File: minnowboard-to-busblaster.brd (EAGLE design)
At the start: 72.4 x 35.6 mm, 19 parts, among them J1 CIRCUITCO_MINNOW2_HIGH_SPEED, U1 SN74LV4T125, U2 SN74LV1T125, U3 SN74LV1T125

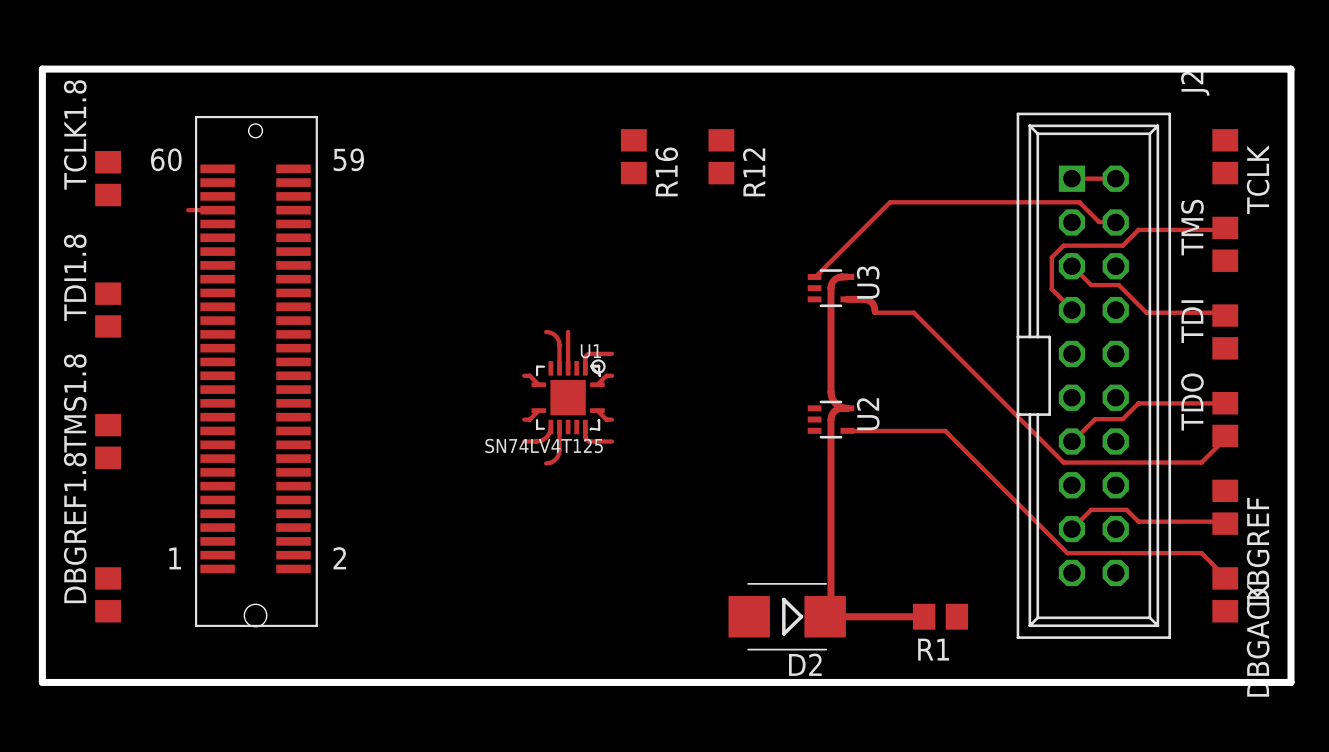
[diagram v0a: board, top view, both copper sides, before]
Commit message: all
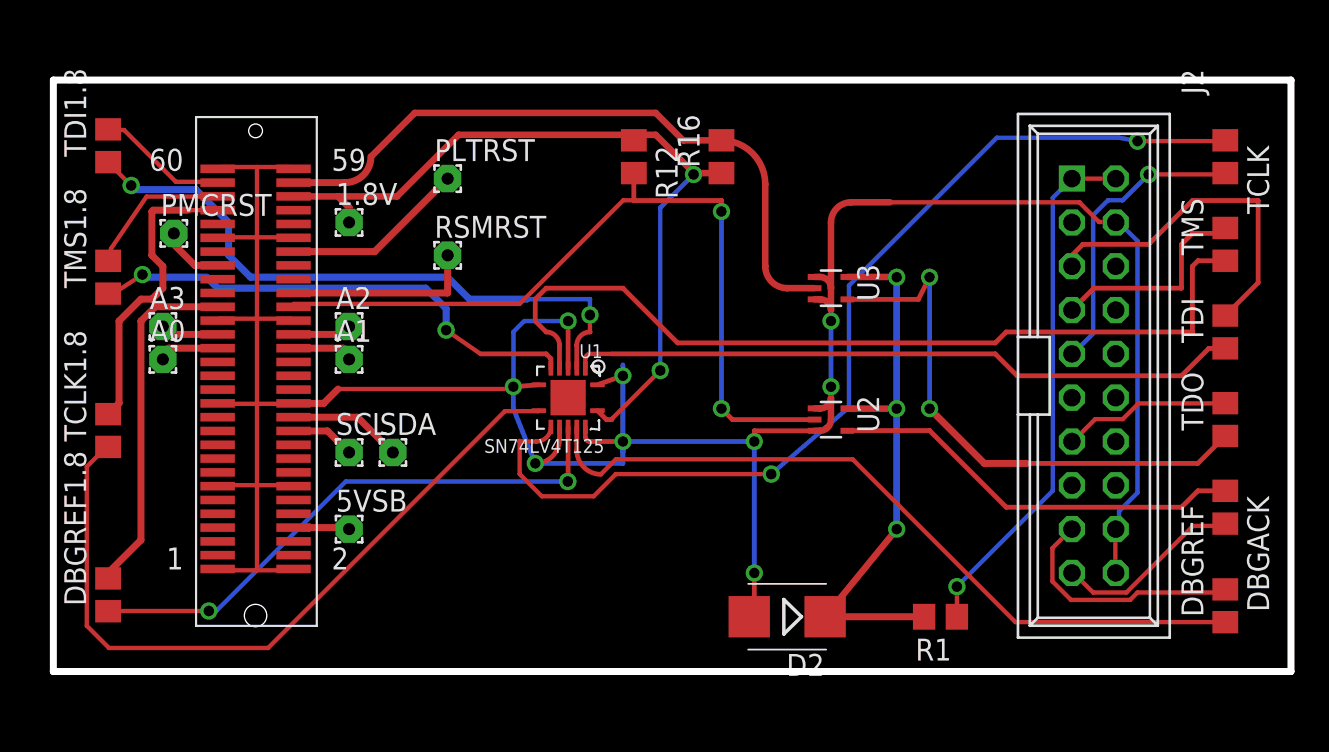
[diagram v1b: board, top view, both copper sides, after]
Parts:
- added 1.8V, 5VSB, A0, A1, A2, A3, PLTRST, PMCRST, RSMRST, SCL, SDA: PAD-TESTPOINT, minnowboard:1,6/0,8
- moved TCLK1.8 14.6 mm to (3.81, 19.7)
- moved TDI1.8 9.52 mm to (3.81, 36.2)
- moved TMS1.8 9.52 mm to (3.81, 28.6)
- moved DBGREF 5.71 mm to (68.6, 9.53), turned to 90 degrees
- moved DBGACK 5.08 mm to (68.6, 15.2)
- moved R12 5.08 mm to (34.3, 35.6)
- moved R16 5.08 mm to (39.4, 35.6), turned to 90 degrees
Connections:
- new net N$11: A1.1, J1.33
- new net N$13: J1.41, RSMRST.1
- new net N$14: A3.1, J1.36
- new net N$15: J1.21, SCL.1
- new net N$16: J1.23, SDA.1
- new net N$7: 5VSB.1, J1.7
- new net N$8: A2.1, J1.35
- new net N$9: A0.1, J1.34
- net +1V8: now also 1.8V.1
- net GND: now also J2.18, J2.20
- net N$23: now also J1.46, PMCRST.1; no longer J2.18
- net N$24: now also J1.47, PLTRST.1; no longer J2.20
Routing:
- net GND: track 28.7 -> 174.6 mm, vias 0 -> 9
- net BB_TCLK_R: track 1.89 -> 58.1 mm, vias 0 -> 2
- net BB_TMS_R: track 2.43 -> 50.4 mm
- net DBGACK: track 0.00 -> 46.8 mm, vias 0 -> 2
- net +1V8: track 1.06 -> 46.9 mm, vias 0 -> 2
- net BB_DBGREQ_R: track 0.00 -> 43.8 mm
- net N$5: track 1.06 -> 43.4 mm
- net TDO: track 0.00 -> 38.9 mm
- net BB_TDI_R: track 2.22 -> 39.0 mm
- net N$4: track 0.00 -> 36.7 mm, vias 0 -> 2
- net N$6: track 0.00 -> 33.2 mm, vias 0 -> 2
- net N$3: track 0.00 -> 29.4 mm, vias 0 -> 2
- net N$1: track 2.54 -> 30.7 mm, vias 0 -> 1
- net DBGREQ: track 0.00 -> 20.2 mm
- net BB_TCLK: track 0.00 -> 17.2 mm, vias 0 -> 1
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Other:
- board size 72.4 x 35.6 mm -> 71.8 x 34.3 mm

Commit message: all
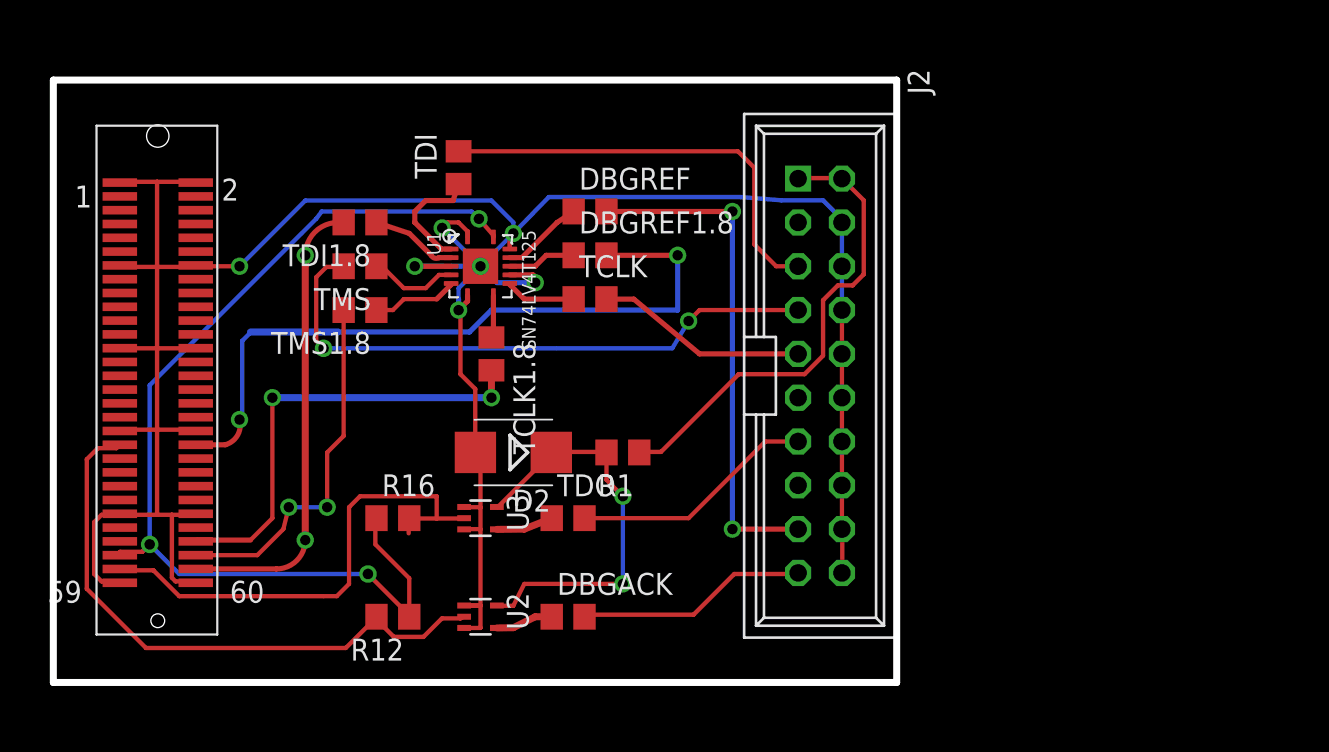
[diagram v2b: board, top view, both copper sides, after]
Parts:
- removed 1.8V, 5VSB, A0, A1, A2, A3, PLTRST, PMCRST, RSMRST, SCL, SDA: PAD-TESTPOINT, minnowboard:1,6/0,8
- moved TMS 50.2 mm to (18.4, 29.2), turned to 180 degrees
- moved TDI 45.5 mm to (24.1, 34.9)
- moved DBGREF 43.3 mm to (31.8, 32.4), turned to 0 degrees
- moved DBGACK 38.6 mm to (30.5, 8.89), turned to 0 degrees
- moved TDO 38.5 mm to (30.5, 14.6), turned to 0 degrees
- moved TCLK 37.7 mm to (31.8, 27.3), turned to 0 degrees
- moved DBGREF1.8 34.2 mm to (31.8, 29.8), turned to 0 degrees
- moved R12 30.1 mm to (20.3, 8.89), turned to 180 degrees
- moved R16 28.3 mm to (20.3, 14.6), turned to 0 degrees
- moved U3 24.3 mm to (25.4, 14.6)
- moved U2 23.3 mm to (25.4, 8.89)
- moved TCLK1.8 22.7 mm to (26.0, 24.1), turned to 270 degrees
- moved R1 20.7 mm to (33.7, 18.4)
- moved D2 18.5 mm to (27.3, 18.4)
- moved J2 15.9 mm to (45.1, 22.9)
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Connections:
- net +1V8: no longer 1.8V.1
- net N$11: no longer A1.1
- net N$13: no longer RSMRST.1
- net N$14: no longer A3.1
- net N$15: no longer SCL.1
- net N$16: no longer SDA.1
- net N$23: no longer PMCRST.1
- net N$24: no longer PLTRST.1
- net N$7: no longer 5VSB.1
- net N$8: no longer A2.1
- net N$9: no longer A0.1
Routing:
- net BB_TCLK_R: track 58.1 -> 4.11 mm, vias 2 -> 0
- net BB_TMS_R: track 50.4 -> 5.18 mm
- net N$5: track 43.4 -> 2.48 mm
- net BB_DBGREQ_R: track 43.8 -> 4.74 mm
- net BB_TDI_R: track 39.0 -> 6.87 mm
- net N$4: track 36.7 -> 4.98 mm, vias 2 -> 0
- net N$6: track 33.2 -> 3.96 mm, vias 2 -> 0
- net BB_TDO_R: track 32.3 -> 3.30 mm, vias 2 -> 0
- net N$3: track 29.4 -> 5.01 mm, vias 2 -> 0
- net BB_TMS: track 12.3 -> 35.0 mm, vias 0 -> 2
- net DBGREQ: track 20.2 -> 41.4 mm, vias 0 -> 2
- net BB_DBGACK_R: track 24.2 -> 3.33 mm
- net TDI: track 7.62 -> 26.6 mm, vias 0 -> 2
- net BB_DBGREQ: track 14.2 -> 29.5 mm, vias 0 -> 2
- net TMS: track 8.51 -> 21.4 mm, vias 0 -> 2
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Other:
- board size 71.8 x 34.3 mm -> 48.9 x 34.9 mm
